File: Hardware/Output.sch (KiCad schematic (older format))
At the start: 20 parts, among them U4 AD9744, U5 THS3091, U6 THS3091, U7 LM285M-ADJ

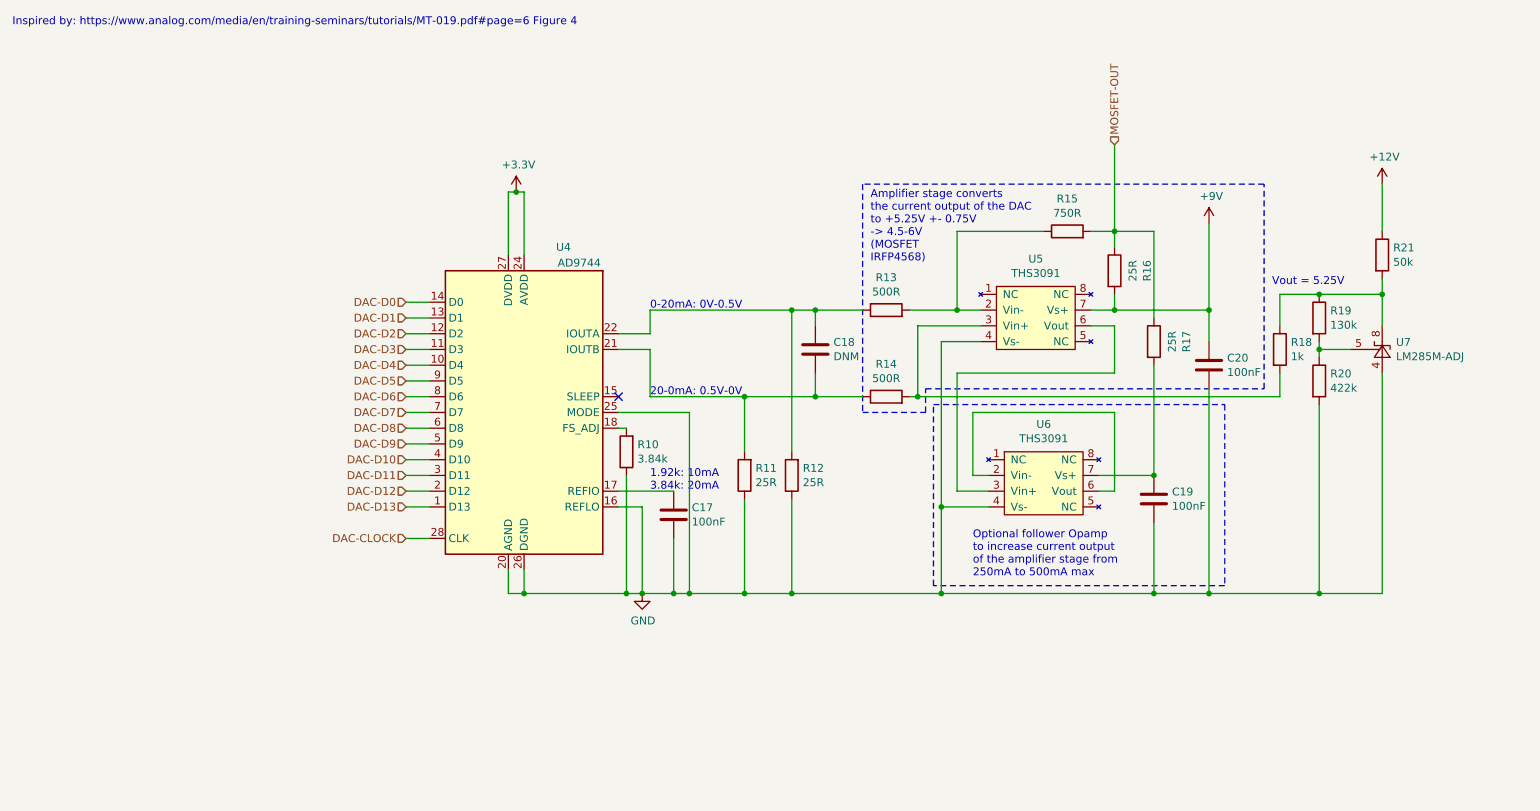
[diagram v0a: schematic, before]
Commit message: fixed output amp biasing
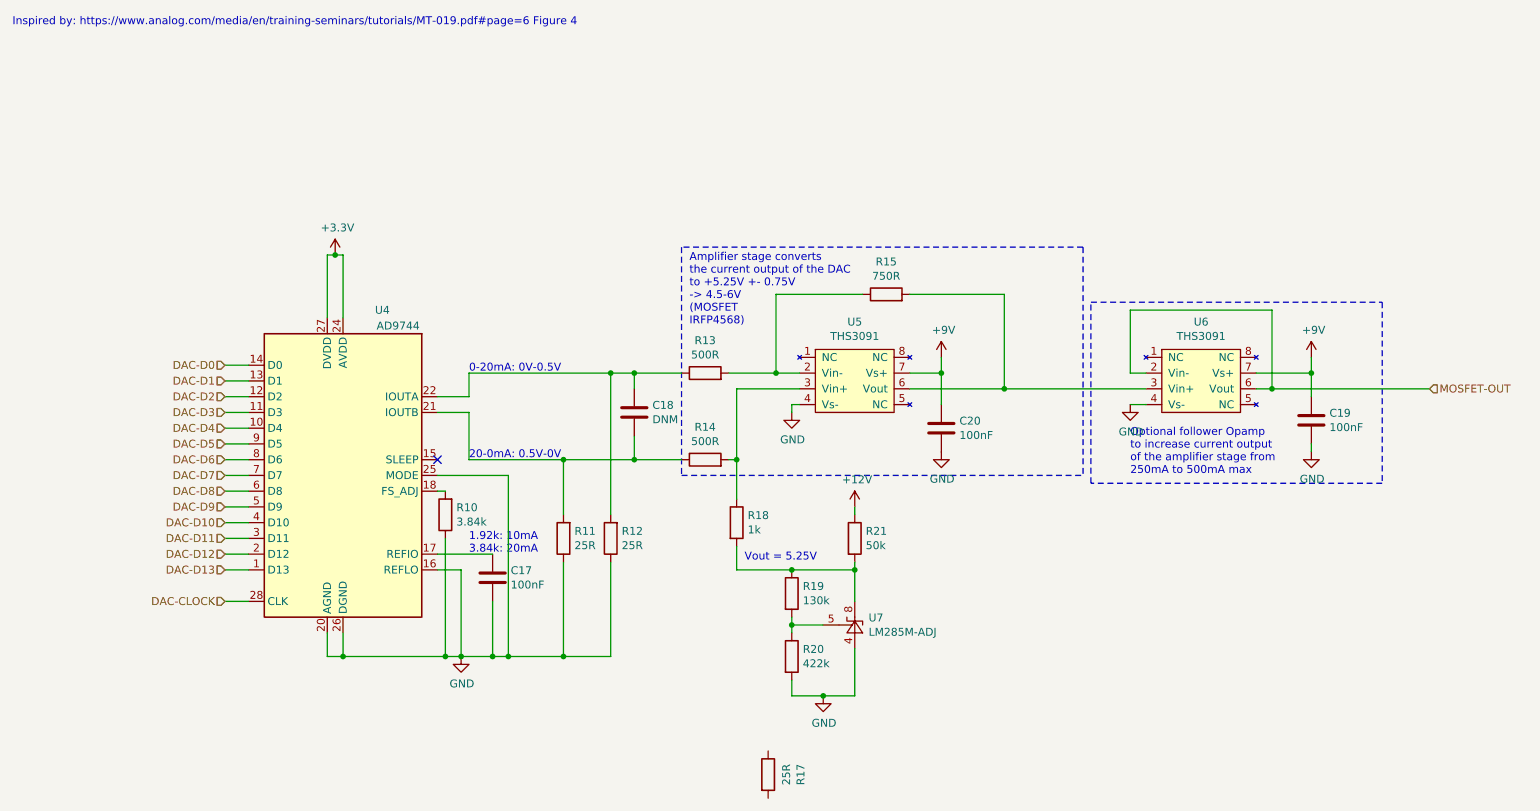
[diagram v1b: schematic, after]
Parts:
- removed R16: 25R, Resistor_SMD:R_0603_1608Metric, symbol Device:R
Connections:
- net +9V: now also C19.2, U6.7 (Vs+)
- net MOSFET-OUT: now also U6.2 (Vin-), U6.6 (Vout); no longer R15.2, R17.1
- net at R14.2, U5.3 (Vin+): now also R18.1; no longer R18.2
- net at U5.6 (Vout), U6.3 (Vin+): now also R15.2
- net at R19.1, R21.2, U7.8 (K): now also R18.2; no longer R18.1
- now unconnected: R17.2
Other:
- moved on the sheet: C17, C18, C19, C20, R10, R11, R12, R13, R14, R15, R17, R18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
